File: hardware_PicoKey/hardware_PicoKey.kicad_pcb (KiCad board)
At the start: 2 copper layers, 36.9 x 18.5 mm, 36 parts, among them J1 USB_A, SW1 SW_Push, SW2 SW_Push, U1 RP2350A-QFN60, U2 AMS1117S-3.3, U3 W25Q128JVS, Y1 Crystal_GND24

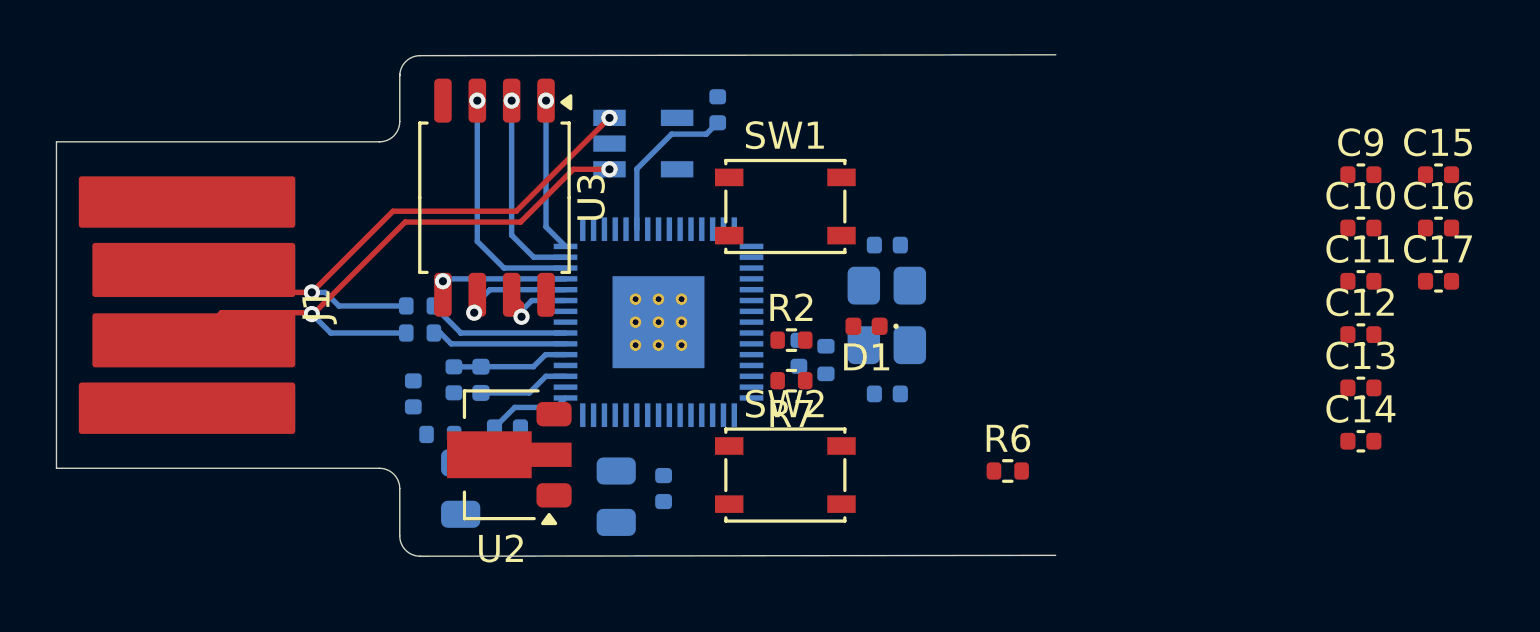
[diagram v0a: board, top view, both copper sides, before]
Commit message: pcb
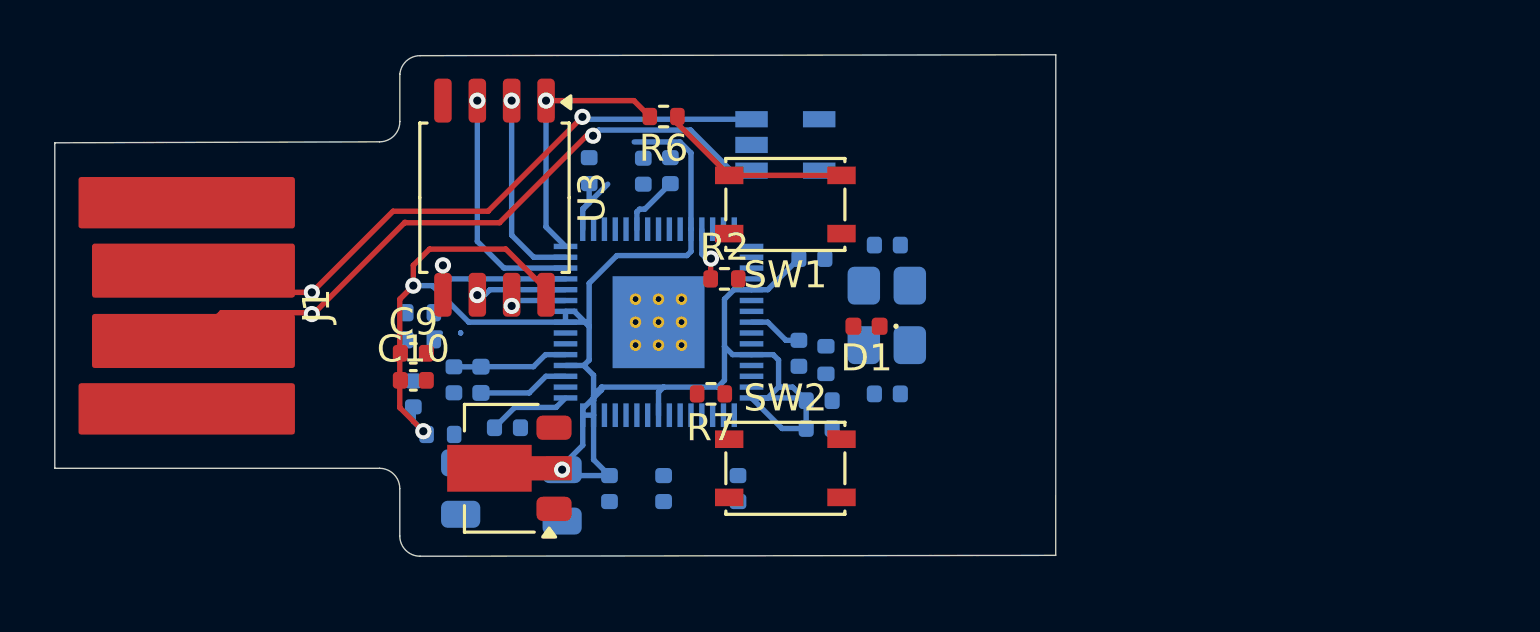
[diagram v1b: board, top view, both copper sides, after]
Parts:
- C11, C12, C13, C14, C15, C16, C17: moved to B.Cu
- moved C9 35.6 mm to (136.2, 70.2)
- moved C10 35.5 mm to (136.2, 71.2)
- moved C16 32.1 mm to (143.5, 75.2), turned to -90 degrees
- moved C15 31.4 mm to (142.8, 63.5), turned to 90 degrees
- moved C17 27.0 mm to (148.2, 75.2), turned to -90 degrees
- moved C11 26.8 mm to (144.8, 63.5), turned to 90 degrees
- moved C12 20.5 mm to (151.0, 66.8)
- moved C13 20.1 mm to (151.2, 73.0)
- moved C14 20.1 mm to (151.2, 72.0)
- moved R6 18.3 mm to (145.5, 61.5), turned to 180 degrees
- moved D2 5.25 mm to (150.0, 62.5)
- moved R2 3.35 mm to (147.8, 67.5)
- moved R7 3.01 mm to (147.2, 71.8)
- moved C6 2.85 mm to (145.8, 63.5)
- moved C5 2.00 mm to (141.8, 75.5)
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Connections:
- R7 pad 1: Net-(U1-GPIO11) -> Net-(U1-GPIO25)
- U1 pad 15: Net-(U1-GPIO11) -> unconnected-(U1-GPIO11-Pad15)
- U1 pad 37: unconnected-(U1-GPIO25-Pad37) -> Net-(U1-GPIO25)
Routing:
- net 3v3: track 0.00 -> 73.9 mm, vias 0 -> 3
- net Net-(R6-Pad1): track 0.00 -> 7.12 mm
- net Net-(U1-USB_DP): track 5.28 -> 0.01 mm
- net Net-(U1-USB_DM): track 5.03 -> 0.24 mm
- net QSPI_SS: track 5.69 -> 9.76 mm
- net USB_DM: track 21.9 -> 24.6 mm
- net Net-(U1-GPIO8): track 0.00 -> 2.08 mm, vias 0 -> 1
- net USB_DP: track 22.1 -> 23.7 mm
- net 1v1: track 10.2 -> 8.65 mm
- net QSPI_SCLK: track 4.59 -> 3.36 mm
- net QSPI_SD0: track 5.07 -> 6.07 mm
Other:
- board size 36.9 x 18.5 mm -> 37 x 18.5 mm
